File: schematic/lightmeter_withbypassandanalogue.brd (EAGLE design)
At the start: 50.7 x 60.4 mm, 54 parts, among them Q1 BSS123, Q2 BSS123, Q3.6 BSS123, Q4.7 BSS123, Q5.8 BSS123, Q6.9 BSS123, Q7.10 BSS123

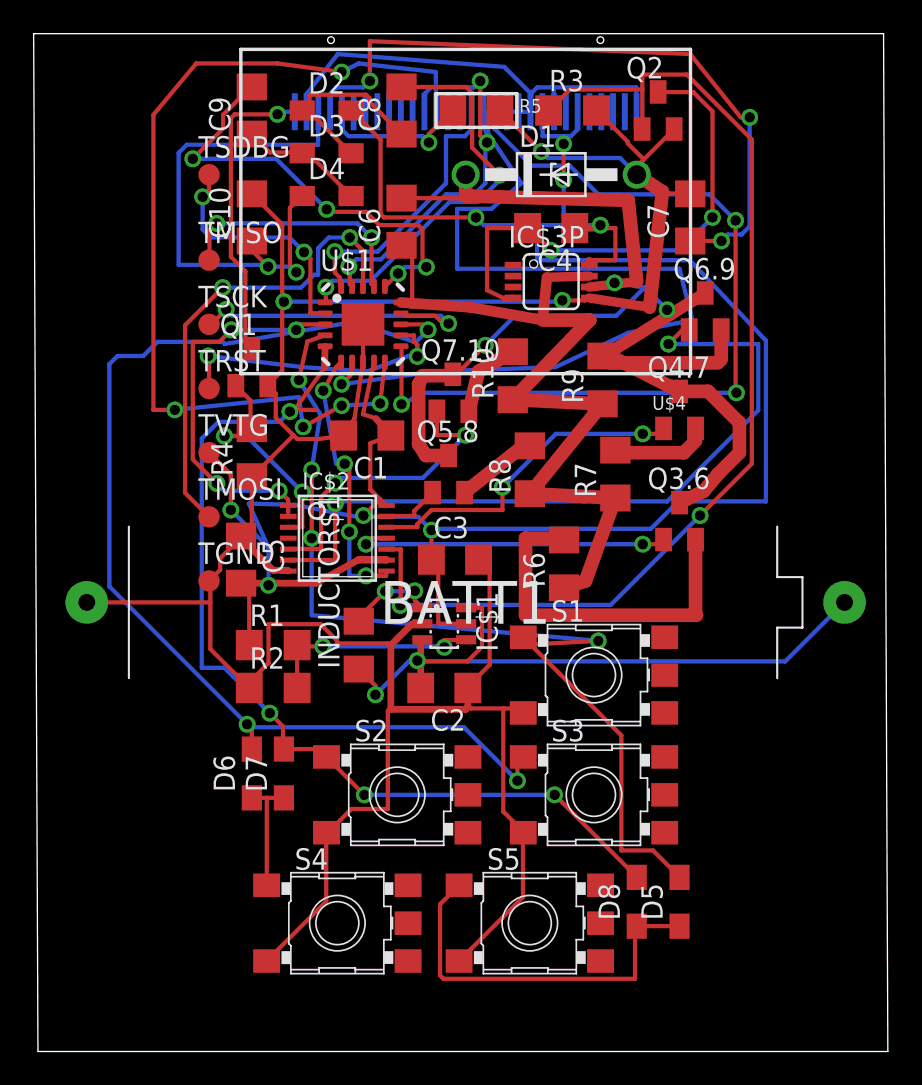
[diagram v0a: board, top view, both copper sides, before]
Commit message: More work on schematic/board.
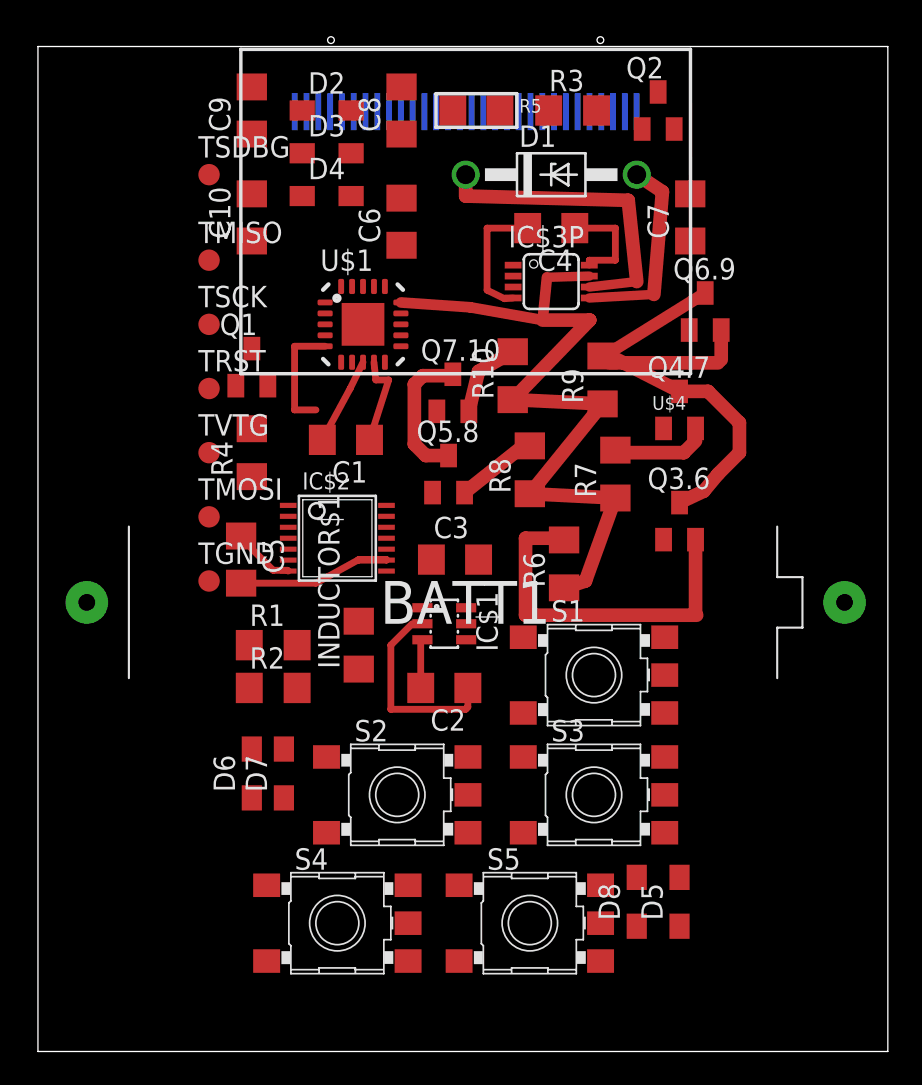
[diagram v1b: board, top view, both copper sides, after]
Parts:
- moved C1 1.30 mm to (37.3, 56.6)
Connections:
- net SCRRES: now also IC$2.4
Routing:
- net GND: track 177.9 -> 32.5 mm, vias 3 -> 0
- net VREG: track 142.3 -> 22.5 mm, vias 8 -> 0
- net PBI$3: track 67.5 -> 0.00 mm, vias 3 -> 0
- net OAPWR: track 65.2 -> 0.00 mm, vias 2 -> 0
- net PBI$1: track 58.2 -> 0.00 mm, vias 4 -> 0
- net SCRCLK: track 56.1 -> 0.00 mm, vias 5 -> 0
- net SCRRES: track 52.1 -> 0.00 mm, vias 1 -> 0
- net SCRCS: track 51.3 -> 0.00 mm, vias 3 -> 0
- net PBI$2: track 57.4 -> 6.86 mm, vias 4 -> 0
- net SCRGRND: track 46.9 -> 0.00 mm, vias 1 -> 0
- net STG$2: track 44.4 -> 0.00 mm, vias 2 -> 0
- net N$25: track 40.9 -> 0.00 mm, vias 3 -> 0
- net VCC: track 42.4 -> 2.90 mm, vias 2 -> 0
- net CPOUT: track 31.2 -> 0.00 mm, vias 2 -> 0
- net AVRMOSI: track 28.1 -> 0.00 mm, vias 2 -> 0
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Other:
- board size 50.7 x 60.4 mm -> 50.5 x 59.7 mm

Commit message: Fix consistency errors and abandon two-layer routing attempt.
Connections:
- net SCRRES: no longer IC$2.4
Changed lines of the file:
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@@
 </signal>
 <signal name="SCRRES">
+<contactref element="U$1" pad="7"/>
 <contactref element="U$4" pad="14"/>
-<contactref element="IC$2" pad="4"/>
-<contactref element="U$1" pad="7"/>
-<wire x1="33.9122" y1="50.8" x2="37.704" y2="61.25" width="0" layer="19" extent="1-1"/>
-<wire x1="45.5" y1="76.13" x2="33.9122" y2="50.8" width="0" layer="19" extent="1-16"/>
+<wire x1="37.704" y1="61.25" x2="45.5" y2="76.13" width="0" layer="19" extent="1-16"/>
 </signal>
 <signal name="N$23">
